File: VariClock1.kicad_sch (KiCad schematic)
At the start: 71 parts, among them U3 40106, U4 4013, U5 40106, U6 40193, U7 TL074, U8 4042, U9 40193

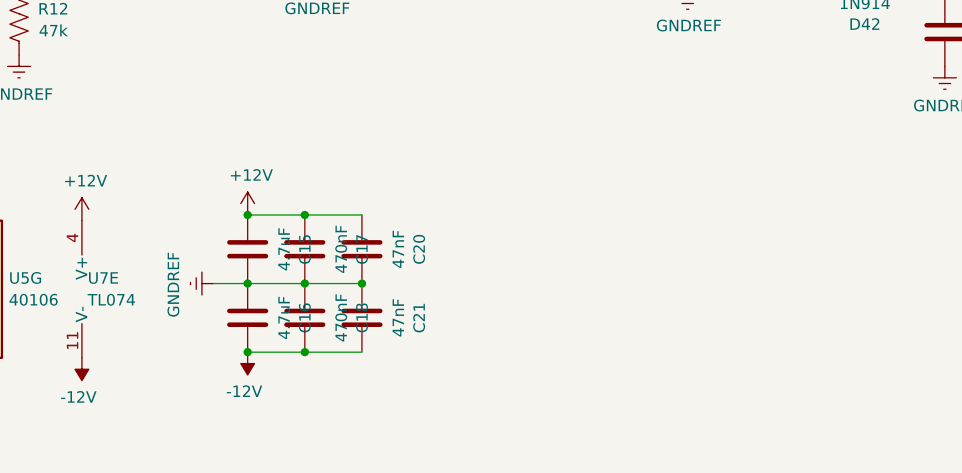
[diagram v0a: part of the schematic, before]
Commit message: routed 100%
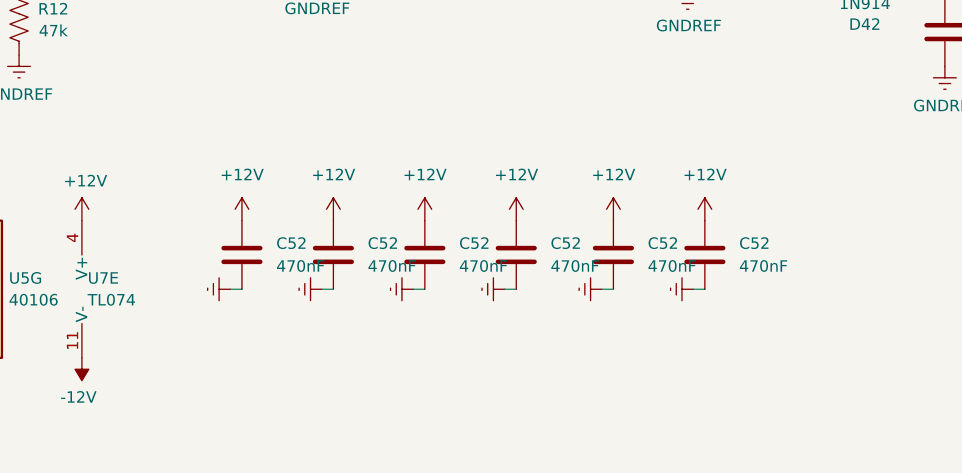
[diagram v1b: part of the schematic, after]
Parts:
- removed C15, C16: 4.7uF, Capacitor_SMD:C_0805_2012Metric, symbol Device:C
- removed C17, C18: 470nF, Capacitor_SMD:C_0805_2012Metric, symbol Device:C
- removed C20, C21: 47nF, Capacitor_SMD:C_0603_1608Metric, symbol Device:C
- added C52 (x6): 470nF, Capacitor_SMD:C_0805_2012Metric, symbol Device:C
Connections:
- net +12V: now also C52.1, C52.1, C52.1, C52.1, C52.1, C52.1
- net GNDREF: now also C52.2, C52.2, C52.2, C52.2, C52.2, C52.2
